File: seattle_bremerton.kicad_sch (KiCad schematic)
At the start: 32 parts

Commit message: single ferry track checkpoint
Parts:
- removed LED419, LED430, LED448, LED449, LED450, LED451, LED452, LED453, LED454, LED455, LED456, LED457, LED461, LED462: WS2812B-2020, EasyEDA:LED-SMD_4P-L2.0-W2.0-TL_WS2812B-2020, symbol EasyEDA:WS2812B-2020

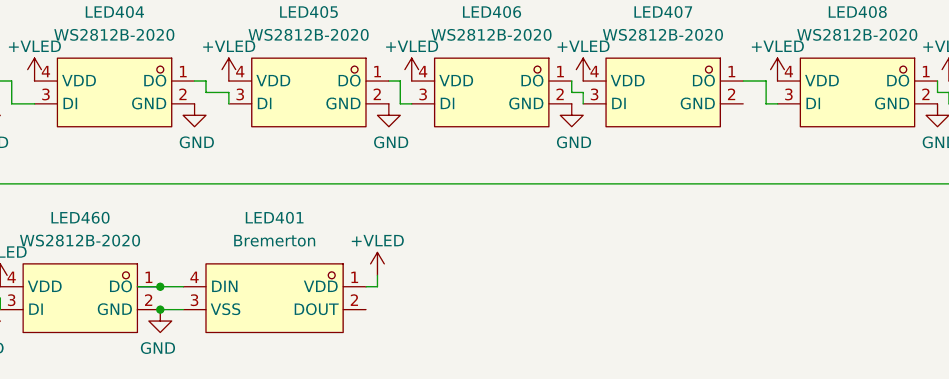
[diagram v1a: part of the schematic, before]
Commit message: checkpoint before label plugin
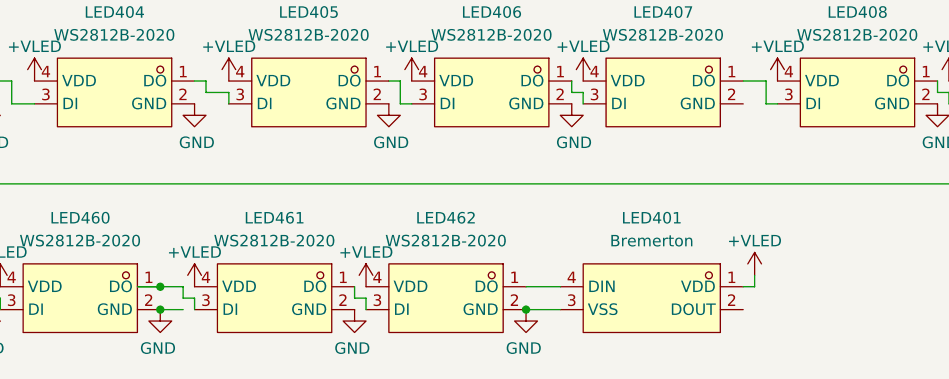
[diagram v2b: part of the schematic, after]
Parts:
- added LED461, LED462: WS2812B-2020, EasyEDA:LED-SMD_4P-L2.0-W2.0-TL_WS2812B-2020, symbol EasyEDA:WS2812B-2020
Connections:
- net +VLED: now also LED461.4 (VDD), LED462.4 (VDD)
- net GND: now also LED461.2 (GND), LED462.2 (GND)
- net at LED460.1 (DO): now also LED461.3 (DI); no longer LED401.4 (DIN)
- new net: LED461.1 (DO), LED462.3 (DI)
- new net: LED401.4 (DIN), LED462.1 (DO)
